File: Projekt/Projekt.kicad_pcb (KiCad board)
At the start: 2 copper layers, 7 parts, among them U1 SHT4x, U2 STM32F446RETx, U3 AMS1117-3.3, U4 PCF8574AP

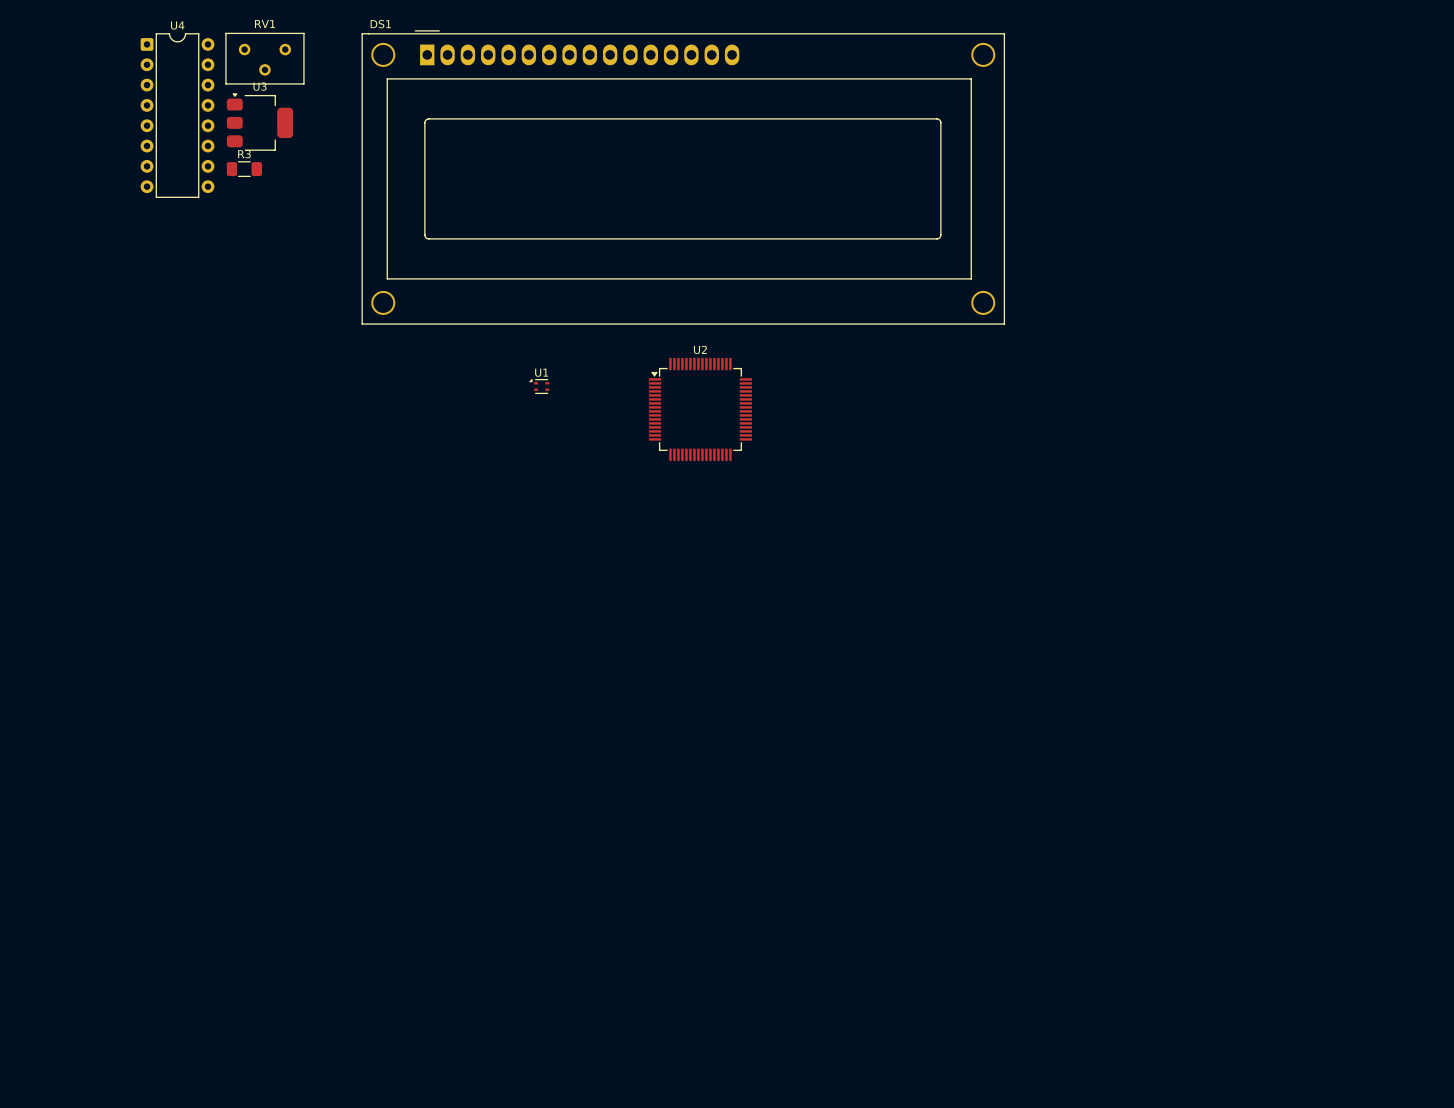
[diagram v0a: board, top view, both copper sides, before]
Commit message: Update
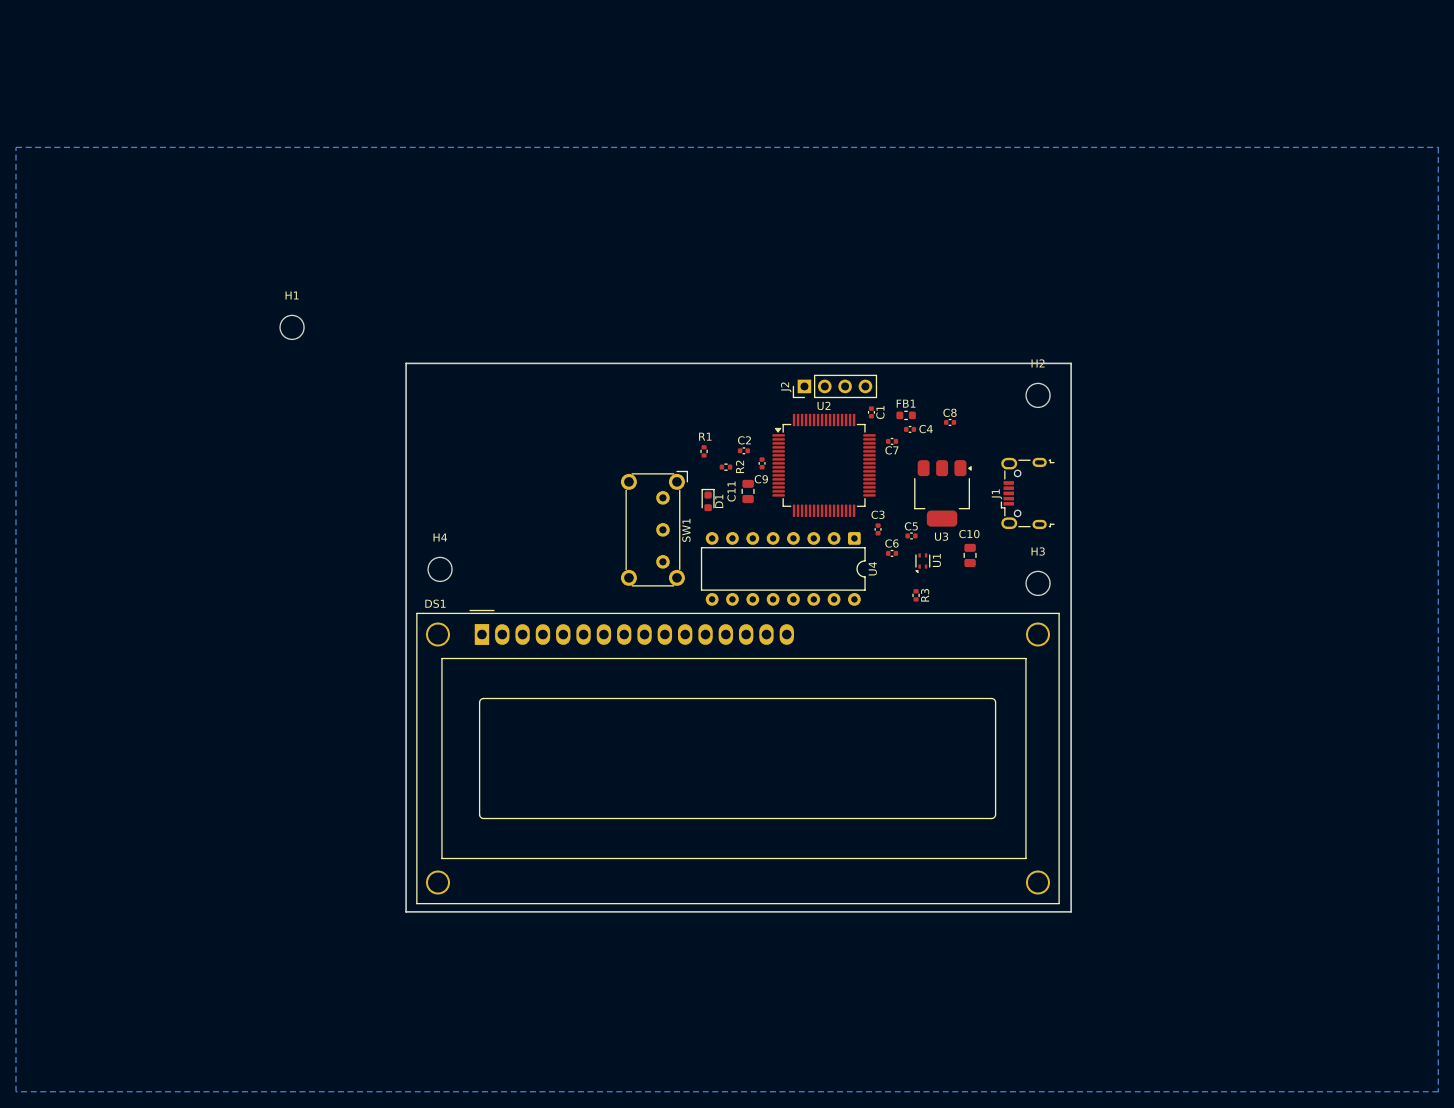
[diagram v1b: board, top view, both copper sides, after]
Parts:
- removed RV1: R_Potentiometer_Small, Potentiometer_THT:Potentiometer_Bourns_3299Y_Vertical
- added C1: 100n, Capacitor_SMD:C_0402_1005Metric, F.Cu at (142.2, 93.1)
- added C10: 22u, Capacitor_SMD:C_0805_2012Metric, F.Cu at (154.5, 111.0)
- added C11: 22u, Capacitor_SMD:C_0805_2012Metric, F.Cu at (126.8, 103.0)
- added C2: 100n, Capacitor_SMD:C_0402_1005Metric, F.Cu at (126.2, 97.9)
- added C3: 100n, Capacitor_SMD:C_0402_1005Metric, F.Cu at (143.0, 107.8)
- added C4: 100n, Capacitor_SMD:C_0402_1005Metric, F.Cu at (147.0, 95.2)
- added C5: 10u, Capacitor_SMD:C_0402_1005Metric, F.Cu at (147.2, 108.6)
- added C6: 10n, Capacitor_SMD:C_0402_1005Metric, F.Cu at (144.8, 110.8)
- added C7: 1u, Capacitor_SMD:C_0402_1005Metric, F.Cu at (144.8, 96.8)
- added C8: 1u, Capacitor_SMD:C_0402_1005Metric, F.Cu at (152.0, 94.4)
- added C9: 100n, Capacitor_SMD:C_0402_1005Metric, F.Cu at (128.5, 99.5)
- added D1: LED, LED_SMD:LED_0603_1608Metric, F.Cu at (121.8, 104.2)
- added FB1: 120 R, Inductor_SMD:L_0603_1608Metric, F.Cu at (146.5, 93.5)
- added H1: MountingHole, MountingHole:MountingHole_3mm, F.Cu at (69.8, 82.5)
- added H2: MountingHole, MountingHole:MountingHole_3mm, F.Cu at (163.0, 91.0)
- added H3: MountingHole, MountingHole:MountingHole_3mm, F.Cu at (163.0, 114.5)
- added H4: MountingHole, MountingHole:MountingHole_3mm, F.Cu at (88.2, 112.8)
- added J1: USB_B_Micro, Connector_USB:USB_Micro-B_Wuerth_629105150521, F.Cu at (161.2, 103.3)
- added J2: Conn_01x04_Pin, Connector_PinHeader_2.54mm:PinHeader_1x04_P2.54mm_Vertical, F.Cu at (133.8, 89.9)
- added R1: 10k, Resistor_SMD:R_0402_1005Metric, F.Cu at (121.2, 98.0)
- added R2: 1k5, Resistor_SMD:R_0402_1005Metric, F.Cu at (124.0, 100.0)
- added SW1: SW_SPDT, Button_Switch_THT:SW_E-Switch_EG1224_SPDT_Angled, F.Cu at (116.1, 103.8)
- R3: footprint Resistor_SMD:R_1206_3216Metric_Pad1.30x1.75mm_HandSolder -> Resistor_SMD:R_0402_1005Metric
- moved U4 107.8 mm to (140.0, 108.9), turned to -90 degrees
- moved R3 99.4 mm to (147.8, 116.0), turned to -90 degrees
- moved U3 97.0 mm to (151.0, 103.2), turned to -90 degrees
- moved DS1 72.8 mm to (93.5, 120.9)
- moved U1 52.4 mm to (148.6, 111.7), turned to 90 degrees
- moved U2 17.0 mm to (136.2, 99.8)
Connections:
- DS1 pad 3: Net-(DS1-VO) -> unconnected-(DS1-VO-Pad3)
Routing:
- added copper zone on B.Cu, net GND
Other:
- board outline added: 83.1 x 68.6 mm
